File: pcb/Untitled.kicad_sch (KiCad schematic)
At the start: 57 parts, among them J1 Conn_01x08_Socket, J2 Micro_SD_Card_Det1, J3 USB_C_Receptacle_USB2.0_14P, J4 Conn_01x02, J5 Conn_Coaxial, Q1 FS8205A, Q2 AO3407A, SW1 reset, SW10 SW_Push, SW2 boot, SW3 SW_Push, SW4 SW_Push, SW5 SW_Push, SW6 SW_Push, SW7 SW_Push, SW8 SW_Push, SW9 SW_Push, U1 ESP32-S3-WROOM-1, U10 RV-3028-C8-32.768KHZ-1PPM-TA-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, U11 BMP390, U2 MAX-M10S, U3 USBLC6-2SC6, U4 MCP73831-2-MC, U5 AP2112K-3.3, U6 DW01A, U8 LIS2MDL, U9 SHT4x

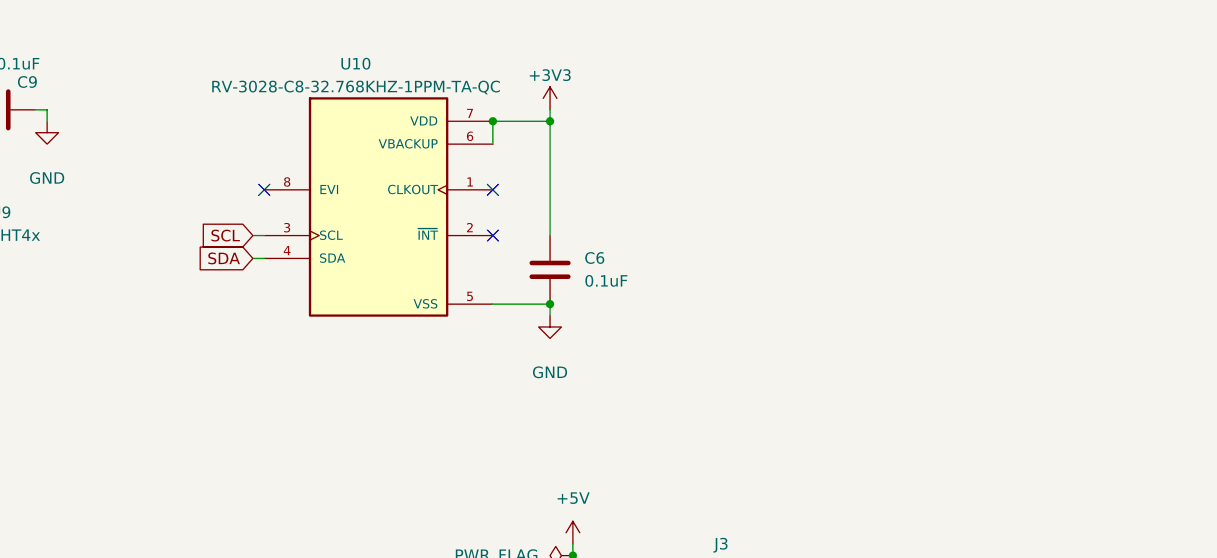
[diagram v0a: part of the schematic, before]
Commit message: update
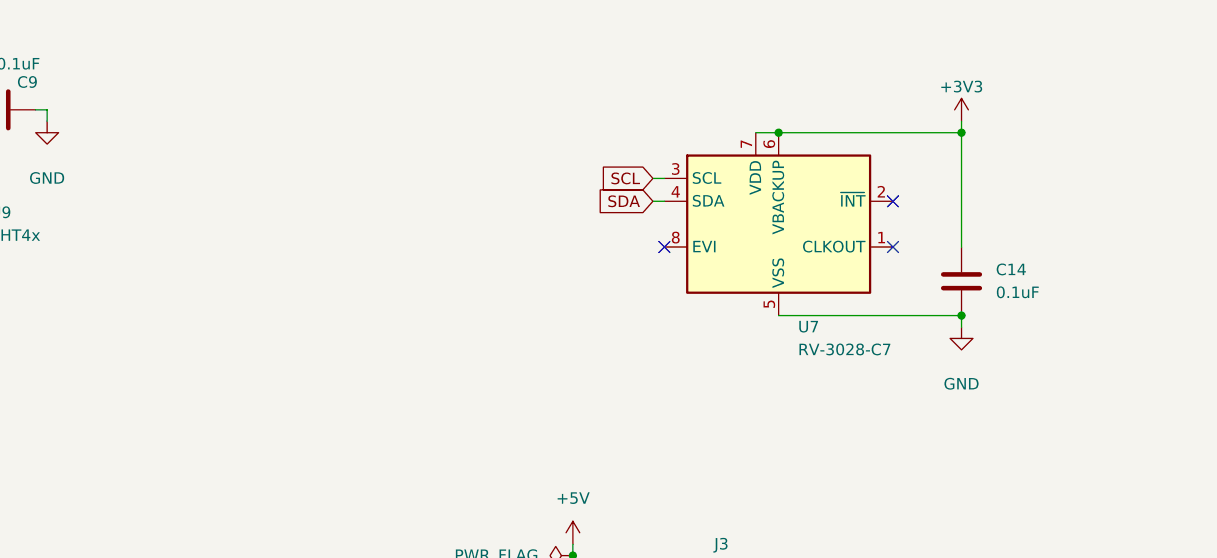
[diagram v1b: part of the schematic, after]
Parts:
- removed C6: 0.1uF, Capacitor_SMD:C_0402_1005Metric, symbol Device:C
- removed U10: RV-3028-C8-32.768KHZ-1PPM-TA-QC, footprintsrv:IC_RV-3028-C8-32.768KHZ-1PPM-TA-QC, symbol RV-3028-C8-32.768KHZ-1PPM-TA-QC:RV-3028-C8-32.768KHZ-1PPM-TA-QC
- added C14: 0.1uF, Capacitor_SMD:C_0402_1005Metric, symbol Device:C
- added U7: RV-3028-C7, Package_SON:MicroCrystal_C7_SON-8_1.5x3.2mm_P0.9mm, symbol Timer_RTC:RV-3028-C7
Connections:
- net +3V3: now also C14.1, U7.6 (VBACKUP), U7.7 (VDD)
- net GND: now also C14.2, U7.5 (VSS)
- net SCL: now also U7.3 (SCL)
- net SDA: now also U7.4 (SDA)
